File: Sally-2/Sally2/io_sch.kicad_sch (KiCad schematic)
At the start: 41 parts, among them J12 Drive 1-4, J13 OPT, J14 Special_Func, J15 TX GND RX, J16 - RI +, J17 RS232, J18 IN RDY CMD OUT GND, J19 Centronics, U10 MAX232, U11 74LS06, U12 74LS06, U13 Z84C30, U14 74LS244, U15 74LS273, U16 74LS244, U8 74LS273, U9 WD1772_PHY

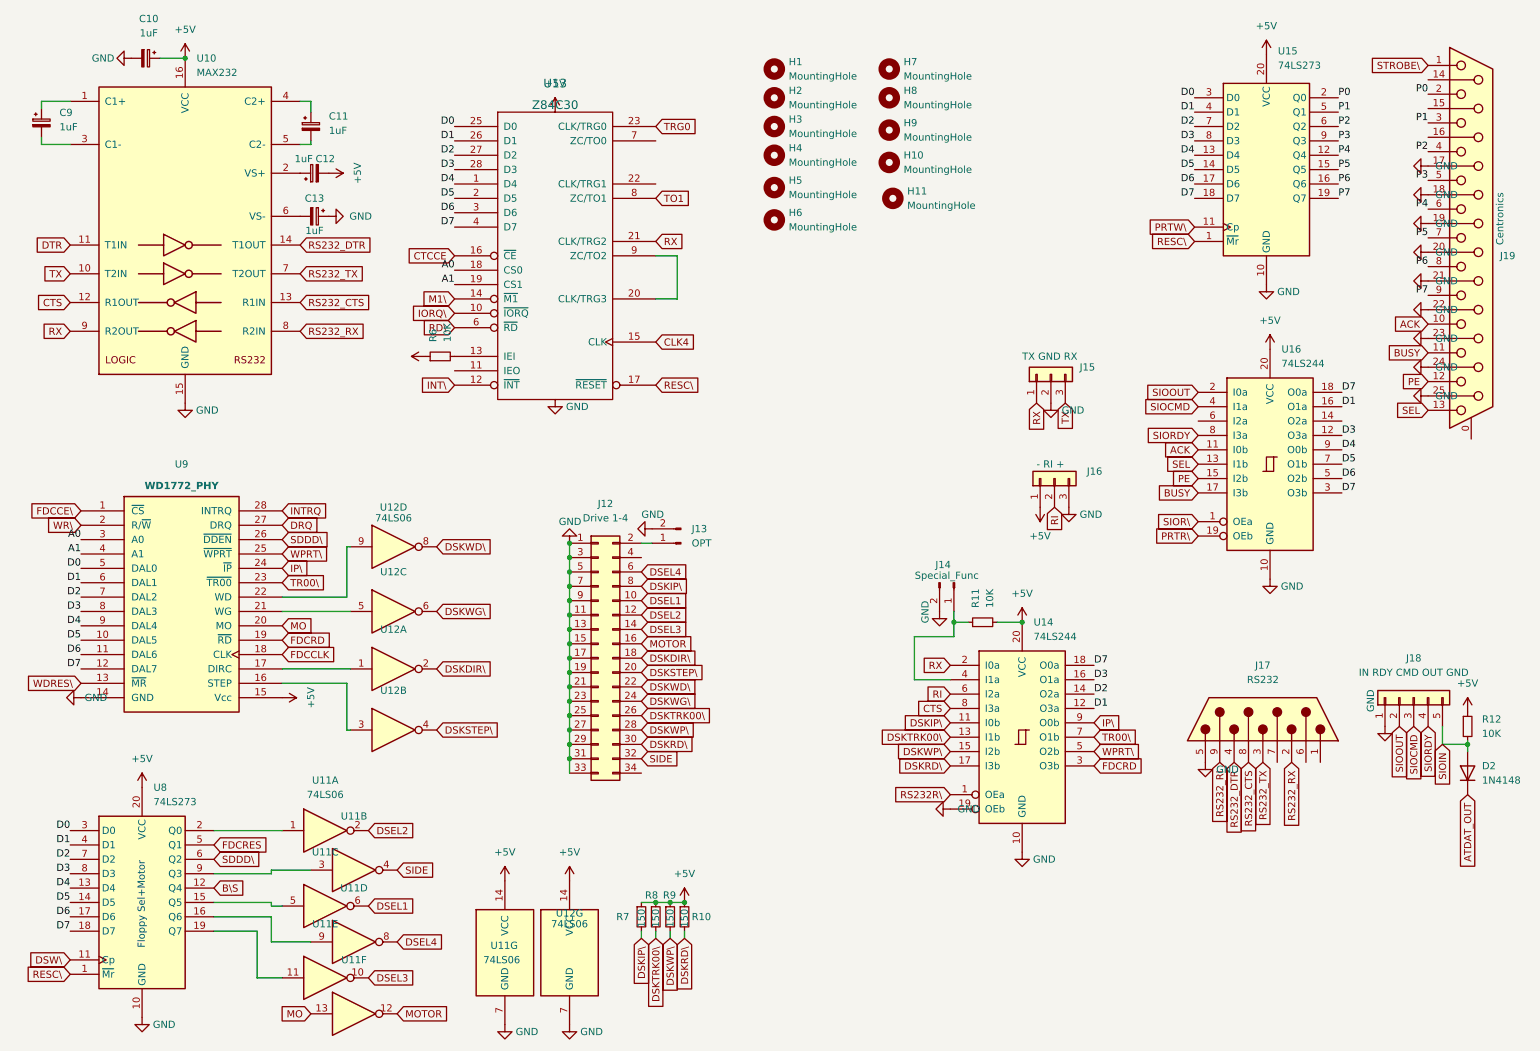
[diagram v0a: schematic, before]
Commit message: workover part 1
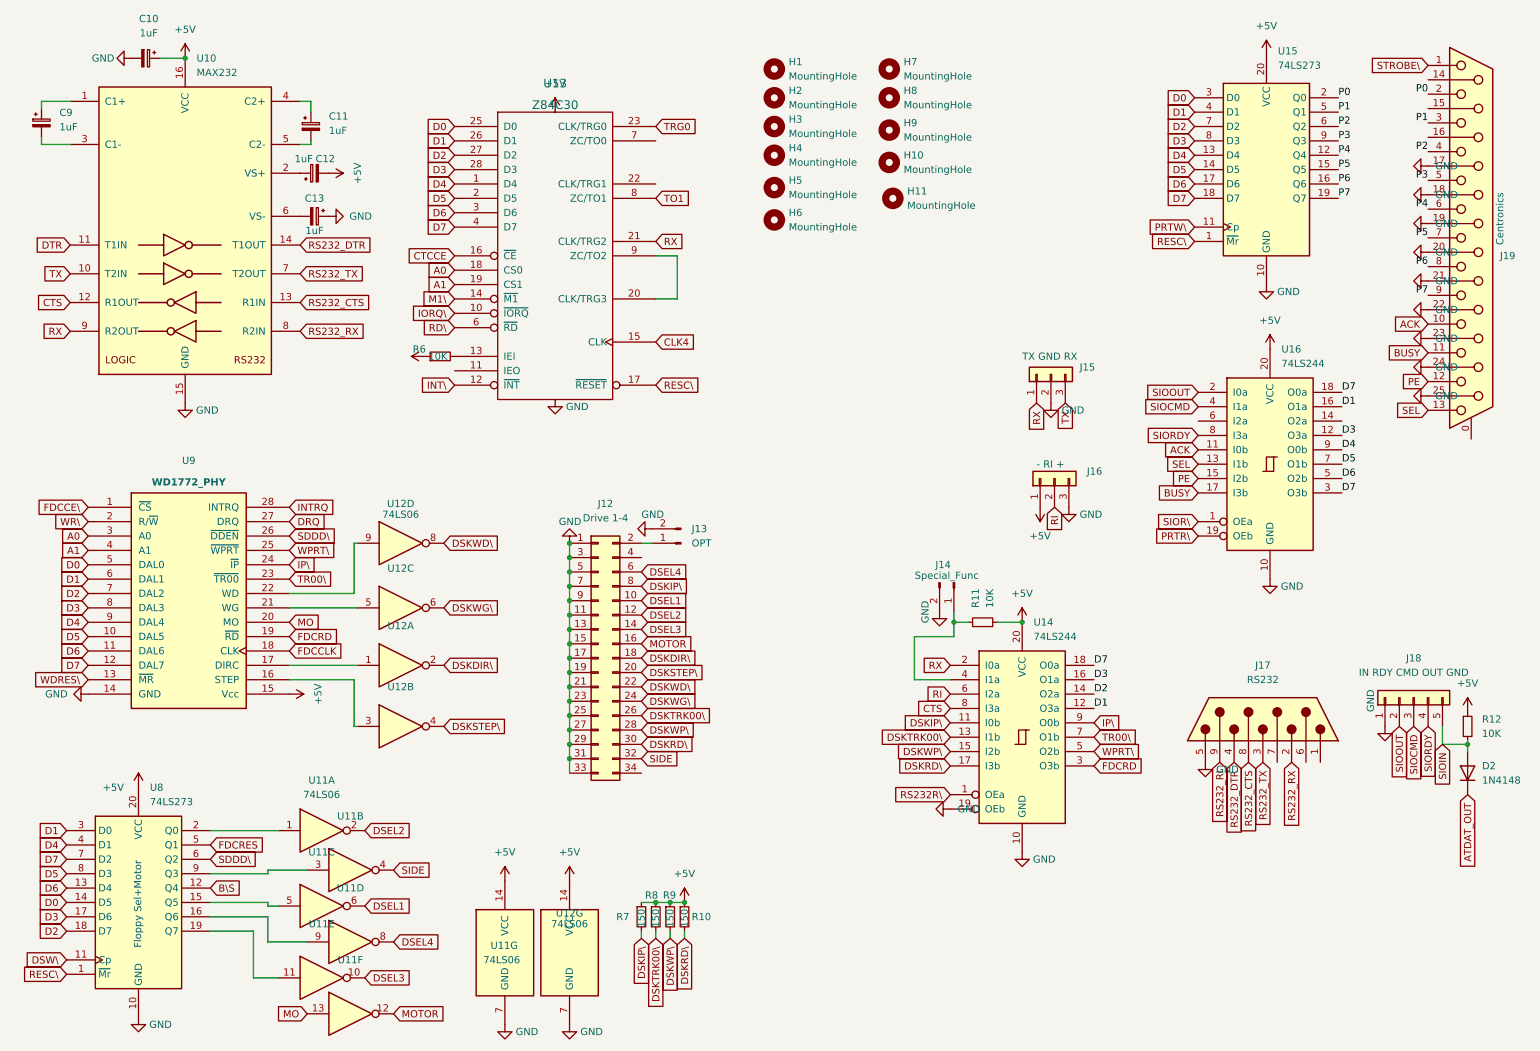
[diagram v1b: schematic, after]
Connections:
- net D0: now also U8.14 (D5); no longer U8.3 (D0)
- net D1: now also U8.3 (D0); no longer U8.4 (D1)
- net D2: now also U8.18 (D7); no longer U8.7 (D2)
- net D3: now also U8.17 (D6); no longer U8.8 (D3)
- net D4: now also U8.4 (D1); no longer U8.13 (D4)
- net D5: now also U8.8 (D3); no longer U8.14 (D5)
- net D6: now also U8.13 (D4); no longer U8.17 (D6)
- net D7: now also U8.7 (D2); no longer U8.18 (D7)
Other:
- moved on the sheet: U11A, U11B, U11C, U11D, U11E, U11F, U12A, U12B, U12C, U12D, U8, U9
